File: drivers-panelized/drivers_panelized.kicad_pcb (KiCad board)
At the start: 2 copper layers, 100.9 x 93.6 mm, 583 parts, among them IC1 Motor_A, IC2 Motor_B, J1 Conn_01x07_Pin, J2 Conn_01x07_Pin

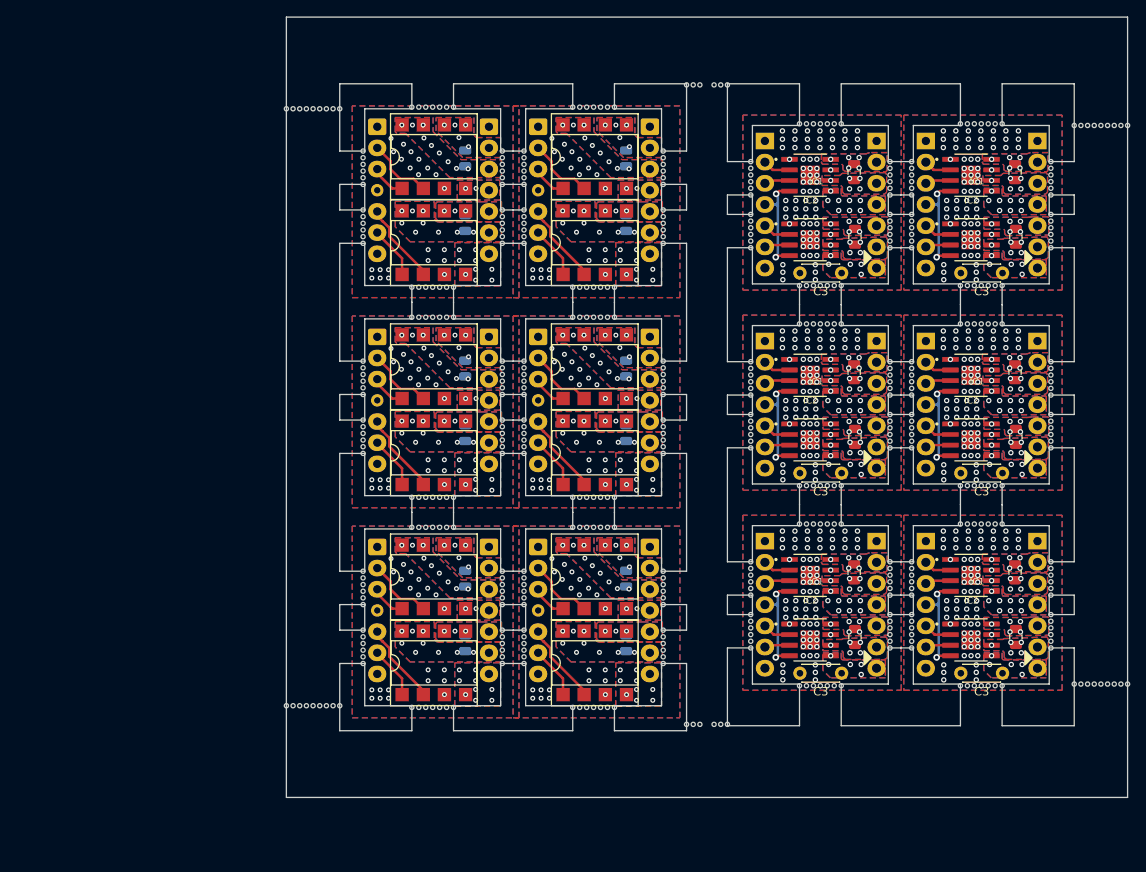
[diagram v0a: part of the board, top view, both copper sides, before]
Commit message: panels again
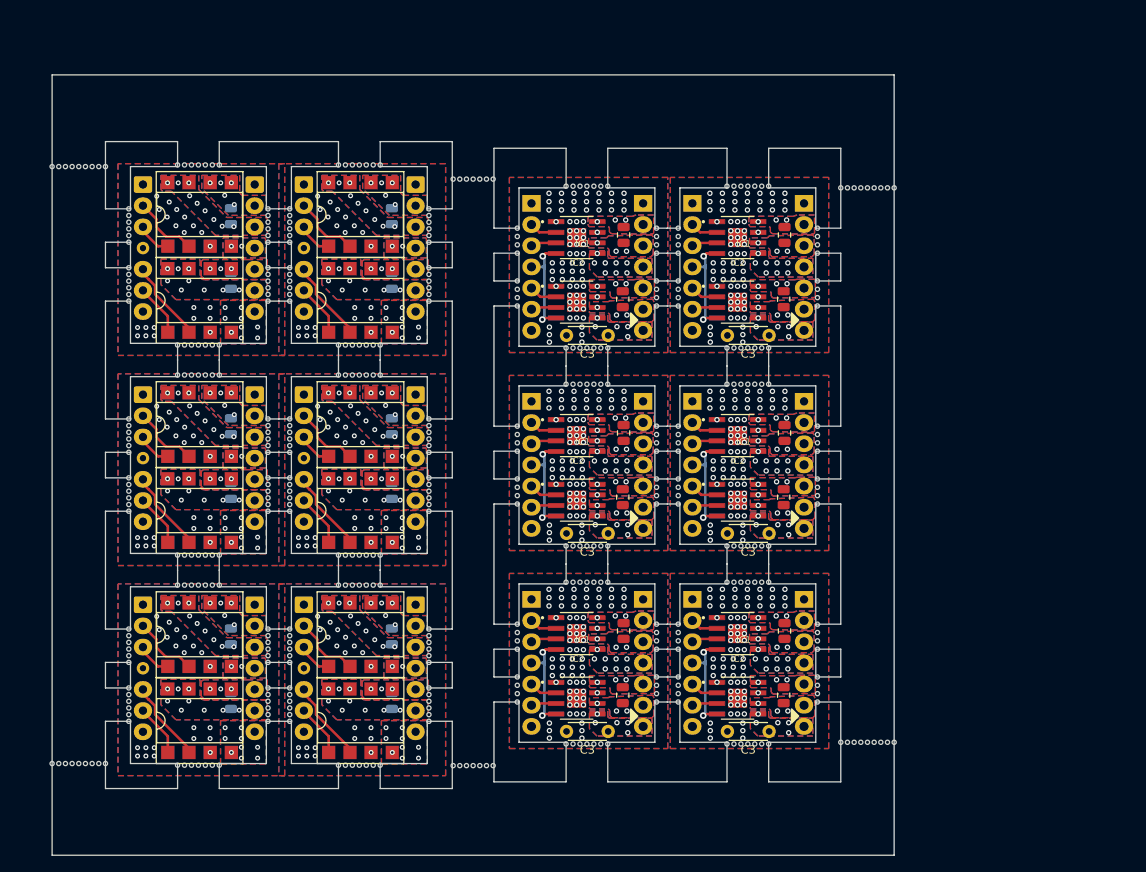
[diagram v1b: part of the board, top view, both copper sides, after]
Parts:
- removed the C1 at (160.3, 97.6)
- removed the C1 at (132.8, 89.4)
- removed the C1 at (113.5, 89.4)
- removed the C1 at (132.8, 64.2)
- removed the C1 at (160.3, 121.6)
- removed the C1 at (179.6, 121.6)
- removed the C1 at (179.6, 73.6)
- removed the C1 at (179.6, 97.6)
- removed the C1 at (160.3, 73.6)
- removed the C1 at (132.8, 114.6)
- removed the C1 at (113.5, 64.2)
- removed the C1 at (113.5, 114.6)
- removed the C2 at (179.5, 65.9)
- removed the C2 at (132.8, 72.0)
- removed the C2 at (113.5, 97.2)
- removed the C2 at (132.8, 97.2)
- removed the C2 at (179.5, 113.9)
- removed the C2 at (179.5, 89.9)
- removed the C2 at (160.2, 89.9)
- removed the C2 at (160.2, 65.9)
- removed the C2 at (160.2, 113.9)
- removed the C2 at (113.5, 122.4)
- removed the C2 at (132.8, 122.4)
- removed the C2 at (113.5, 72.0)
- removed the C3 at (158.7, 78.0)
- removed the C3 at (178.0, 102.0)
- removed the C3 at (178.0, 78.0)
- removed the C3 at (158.7, 126.0)
- removed the C3 at (178.0, 126.0)
- removed the C3 at (158.7, 102.0)
- removed the IC1 at (174.2, 74.0)
- removed the IC1 at (154.9, 74.0)
- removed the IC1 at (174.2, 98.0)
- removed the IC1 at (174.2, 122.0)
- removed the IC1 at (154.9, 98.0)
- removed the IC1 at (154.9, 122.0)
- removed the IC2 at (174.2, 114.2)
- removed the IC2 at (154.9, 90.2)
- removed the IC2 at (174.2, 90.2)
- removed the IC2 at (174.2, 66.2)
- removed the IC2 at (154.9, 114.2)
- removed the IC2 at (154.9, 66.2)
- removed the J1 at (103.0, 60.4)
- removed the J1 at (103.0, 110.8)
- removed the J1 at (149.5, 86.1)
- removed the J1 at (149.5, 110.1)
- removed the J1 at (149.5, 62.1)
- removed the J1 at (168.8, 62.1)
- removed the J1 at (122.3, 60.4)
- removed the J1 at (122.3, 85.6)
- removed the J1 at (168.8, 86.1)
- removed the J1 at (103.0, 85.6)
- removed the J1 at (122.3, 110.8)
- removed the J1 at (168.8, 110.1)
- removed the J2 at (135.7, 85.6)
- removed the J2 at (135.7, 110.8)
- removed the J2 at (162.9, 62.1)
- removed the J2 at (116.4, 85.6)
- removed the J2 at (135.7, 60.4)
- removed the J2 at (162.9, 110.1)
- removed the J2 at (162.9, 86.1)
- removed the J2 at (182.2, 110.1)
- removed the J2 at (182.2, 86.1)
- removed the J2 at (116.4, 60.4)
- removed the J2 at (116.4, 110.8)
- removed the J2 at (182.2, 62.1)
- removed the KiKit_MB_10_1 at (183.8, 70.9)
- removed the KiKit_MB_10_1 at (137.3, 70.4)
- removed the KiKit_MB_10_2 at (183.8, 71.7)
- removed the KiKit_MB_10_2 at (137.3, 71.2)
- removed the KiKit_MB_10_3 at (137.3, 72.0)
- removed the KiKit_MB_10_3 at (183.8, 72.5)
- removed the KiKit_MB_10_4 at (137.3, 72.8)
- removed the KiKit_MB_10_4 at (183.8, 73.3)
- removed the KiKit_MB_10_5 at (137.3, 73.6)
- removed the KiKit_MB_10_5 at (183.8, 74.1)
- removed the KiKit_MB_10_6 at (183.8, 74.9)
- removed the KiKit_MB_10_6 at (137.3, 74.4)
- removed the KiKit_MB_11_1 at (126.5, 58.1)
- removed the KiKit_MB_11_1 at (172.9, 60.1)
- removed the KiKit_MB_11_2 at (173.8, 60.1)
- removed the KiKit_MB_11_2 at (127.3, 58.1)
- removed the KiKit_MB_11_3 at (128.1, 58.1)
- removed the KiKit_MB_11_3 at (174.6, 60.1)
- removed the KiKit_MB_11_4 at (128.9, 58.1)
- removed the KiKit_MB_11_4 at (175.4, 60.1)
- removed the KiKit_MB_11_5 at (129.8, 58.1)
- removed the KiKit_MB_11_5 at (176.3, 60.1)
- removed the KiKit_MB_11_6 at (130.6, 58.1)
- removed the KiKit_MB_11_6 at (177.1, 60.1)
- removed the KiKit_MB_11_7 at (177.9, 60.1)
- removed the KiKit_MB_11_7 at (131.4, 58.1)
- removed the KiKit_MB_12_1 at (131.4, 79.7)
- removed the KiKit_MB_12_1 at (177.9, 79.5)
- removed the KiKit_MB_12_2 at (130.6, 79.7)
- removed the KiKit_MB_12_2 at (177.1, 79.5)
- removed the KiKit_MB_12_3 at (129.8, 79.7)
- removed the KiKit_MB_12_3 at (176.3, 79.5)
- removed the KiKit_MB_12_4 at (175.4, 79.5)
- removed the KiKit_MB_12_4 at (128.9, 79.7)
- removed the KiKit_MB_12_5 at (128.1, 79.7)
- removed the KiKit_MB_12_5 at (174.6, 79.5)
- removed the KiKit_MB_12_6 at (127.3, 79.7)
- removed the KiKit_MB_12_6 at (173.8, 79.5)
- removed the KiKit_MB_12_7 at (126.5, 79.7)
- removed the KiKit_MB_12_7 at (172.9, 79.5)
- removed the KiKit_MB_13_1 at (147.8, 92.6)
- removed the KiKit_MB_13_1 at (101.3, 92.5)
- removed the KiKit_MB_13_2 at (147.8, 91.8)
- removed the KiKit_MB_13_2 at (101.3, 91.7)
- removed the KiKit_MB_13_3 at (101.3, 90.9)
- removed the KiKit_MB_13_3 at (147.8, 91.0)
- removed the KiKit_MB_13_4 at (101.3, 90.1)
- removed the KiKit_MB_13_4 at (147.8, 90.2)
- removed the KiKit_MB_13_5 at (147.8, 89.4)
- removed the KiKit_MB_13_5 at (101.3, 89.3)
- removed the KiKit_MB_13_6 at (101.3, 88.5)
- removed the KiKit_MB_13_6 at (147.8, 88.6)
- removed the KiKit_MB_14_1 at (101.3, 99.6)
- removed the KiKit_MB_14_1 at (147.8, 98.9)
- removed the KiKit_MB_14_2 at (147.8, 98.1)
- removed the KiKit_MB_14_2 at (101.3, 98.8)
- removed the KiKit_MB_14_3 at (101.3, 98.0)
- removed the KiKit_MB_14_3 at (147.8, 97.3)
- removed the KiKit_MB_14_4 at (101.3, 97.2)
- removed the KiKit_MB_14_4 at (147.8, 96.5)
- removed the KiKit_MB_14_5 at (101.3, 96.4)
- removed the KiKit_MB_14_5 at (147.8, 95.7)
- removed the KiKit_MB_14_6 at (147.8, 94.9)
- removed the KiKit_MB_14_6 at (101.3, 95.6)
- removed the KiKit_MB_15_1 at (118.0, 88.5)
- removed the KiKit_MB_15_1 at (164.5, 88.6)
- removed the KiKit_MB_15_2 at (118.0, 89.3)
- removed the KiKit_MB_15_2 at (164.5, 89.4)
- removed the KiKit_MB_15_3 at (164.5, 90.2)
- removed the KiKit_MB_15_3 at (118.0, 90.1)
- removed the KiKit_MB_15_4 at (164.5, 91.0)
- removed the KiKit_MB_15_4 at (118.0, 90.9)
- removed the KiKit_MB_15_5 at (164.5, 91.8)
- removed the KiKit_MB_15_5 at (118.0, 91.7)
- removed the KiKit_MB_15_6 at (118.0, 92.5)
- removed the KiKit_MB_15_6 at (164.5, 92.6)
- removed the KiKit_MB_16_1 at (164.5, 94.9)
- removed the KiKit_MB_16_1 at (118.0, 95.6)
- removed the KiKit_MB_16_2 at (118.0, 96.4)
- removed the KiKit_MB_16_2 at (164.5, 95.7)
- removed the KiKit_MB_16_3 at (164.5, 96.5)
- removed the KiKit_MB_16_3 at (118.0, 97.2)
- removed the KiKit_MB_16_4 at (118.0, 98.0)
- removed the KiKit_MB_16_4 at (164.5, 97.3)
- removed the KiKit_MB_16_5 at (118.0, 98.8)
- removed the KiKit_MB_16_5 at (164.5, 98.1)
- removed the KiKit_MB_16_6 at (118.0, 99.6)
- removed the KiKit_MB_16_6 at (164.5, 98.9)
- removed the KiKit_MB_17_1 at (107.2, 83.3)
- removed the KiKit_MB_17_1 at (153.7, 84.1)
- removed the KiKit_MB_17_2 at (108.0, 83.3)
- removed the KiKit_MB_17_2 at (154.5, 84.1)
- removed the KiKit_MB_17_3 at (108.8, 83.3)
- removed the KiKit_MB_17_3 at (155.3, 84.1)
- removed the KiKit_MB_17_4 at (156.2, 84.1)
- removed the KiKit_MB_17_4 at (109.7, 83.3)
- removed the KiKit_MB_17_5 at (110.5, 83.3)
- removed the KiKit_MB_17_5 at (157.0, 84.1)
- removed the KiKit_MB_17_6 at (111.3, 83.3)
- removed the KiKit_MB_17_6 at (157.8, 84.1)
- removed the KiKit_MB_17_7 at (112.2, 83.3)
- removed the KiKit_MB_17_7 at (158.7, 84.1)
- removed the KiKit_MB_18_1 at (112.2, 104.9)
- removed the KiKit_MB_18_1 at (158.7, 103.5)
- removed the KiKit_MB_18_2 at (111.3, 104.9)
- removed the KiKit_MB_18_2 at (157.8, 103.5)
- removed the KiKit_MB_18_3 at (110.5, 104.9)
- removed the KiKit_MB_18_3 at (157.0, 103.5)
- removed the KiKit_MB_18_4 at (156.2, 103.5)
- removed the KiKit_MB_18_4 at (109.7, 104.9)
- removed the KiKit_MB_18_5 at (155.3, 103.5)
- removed the KiKit_MB_18_5 at (108.8, 104.9)
- removed the KiKit_MB_18_6 at (108.0, 104.9)
- removed the KiKit_MB_18_6 at (154.5, 103.5)
- removed the KiKit_MB_18_7 at (107.2, 104.9)
- removed the KiKit_MB_18_7 at (153.7, 103.5)
- removed the KiKit_MB_19_1 at (167.1, 92.6)
- removed the KiKit_MB_19_1 at (120.6, 92.5)
- removed the KiKit_MB_19_2 at (120.6, 91.7)
- removed the KiKit_MB_19_2 at (167.1, 91.8)
- removed the KiKit_MB_19_3 at (167.1, 91.0)
- removed the KiKit_MB_19_3 at (120.6, 90.9)
- removed the KiKit_MB_19_4 at (167.1, 90.2)
- removed the KiKit_MB_19_4 at (120.6, 90.1)
- removed the KiKit_MB_19_5 at (167.1, 89.4)
- removed the KiKit_MB_19_5 at (120.6, 89.3)
- removed the KiKit_MB_19_6 at (167.1, 88.6)
- removed the KiKit_MB_19_6 at (120.6, 88.5)
- removed the KiKit_MB_1_1 at (101.3, 67.3)
- removed the KiKit_MB_1_1 at (147.8, 68.6)
- removed the KiKit_MB_1_2 at (101.3, 66.5)
- removed the KiKit_MB_1_2 at (147.8, 67.8)
- removed the KiKit_MB_1_3 at (101.3, 65.7)
- removed the KiKit_MB_1_3 at (147.8, 67.0)
- removed the KiKit_MB_1_4 at (101.3, 64.9)
- removed the KiKit_MB_1_4 at (147.8, 66.2)
- removed the KiKit_MB_1_5 at (101.3, 64.1)
- removed the KiKit_MB_1_5 at (147.8, 65.4)
- removed the KiKit_MB_1_6 at (147.8, 64.6)
- removed the KiKit_MB_1_6 at (101.3, 63.3)
- removed the KiKit_MB_20_1 at (120.6, 99.6)
- removed the KiKit_MB_20_1 at (167.1, 98.9)
- removed the KiKit_MB_20_2 at (167.1, 98.1)
- removed the KiKit_MB_20_2 at (120.6, 98.8)
- removed the KiKit_MB_20_3 at (120.6, 98.0)
- removed the KiKit_MB_20_3 at (167.1, 97.3)
- removed the KiKit_MB_20_4 at (120.6, 97.2)
- removed the KiKit_MB_20_4 at (167.1, 96.5)
- removed the KiKit_MB_20_5 at (120.6, 96.4)
- removed the KiKit_MB_20_5 at (167.1, 95.7)
- removed the KiKit_MB_20_6 at (167.1, 94.9)
- removed the KiKit_MB_20_6 at (120.6, 95.6)
- removed the KiKit_MB_21_1 at (183.8, 88.6)
- removed the KiKit_MB_21_1 at (137.3, 88.5)
- removed the KiKit_MB_21_2 at (183.8, 89.4)
- removed the KiKit_MB_21_2 at (137.3, 89.3)
- removed the KiKit_MB_21_3 at (137.3, 90.1)
- removed the KiKit_MB_21_3 at (183.8, 90.2)
- removed the KiKit_MB_21_4 at (183.8, 91.0)
- removed the KiKit_MB_21_4 at (137.3, 90.9)
- removed the KiKit_MB_21_5 at (183.8, 91.8)
- removed the KiKit_MB_21_5 at (137.3, 91.7)
- removed the KiKit_MB_21_6 at (183.8, 92.6)
- removed the KiKit_MB_21_6 at (137.3, 92.5)
- removed the KiKit_MB_22_1 at (183.8, 94.9)
- removed the KiKit_MB_22_1 at (137.3, 95.6)
- removed the KiKit_MB_22_2 at (183.8, 95.7)
- removed the KiKit_MB_22_2 at (137.3, 96.4)
- removed the KiKit_MB_22_3 at (183.8, 96.5)
- removed the KiKit_MB_22_3 at (137.3, 97.2)
- removed the KiKit_MB_22_4 at (137.3, 98.0)
- removed the KiKit_MB_22_4 at (183.8, 97.3)
- removed the KiKit_MB_22_5 at (137.3, 98.8)
- removed the KiKit_MB_22_5 at (183.8, 98.1)
- removed the KiKit_MB_22_6 at (183.8, 98.9)
- removed the KiKit_MB_22_6 at (137.3, 99.6)
- removed the KiKit_MB_23_1 at (172.9, 84.1)
- removed the KiKit_MB_23_1 at (126.5, 83.3)
- removed the KiKit_MB_23_2 at (173.8, 84.1)
- removed the KiKit_MB_23_2 at (127.3, 83.3)
- removed the KiKit_MB_23_3 at (174.6, 84.1)
- removed the KiKit_MB_23_3 at (128.1, 83.3)
- removed the KiKit_MB_23_4 at (175.4, 84.1)
- removed the KiKit_MB_23_4 at (128.9, 83.3)
- removed the KiKit_MB_23_5 at (176.3, 84.1)
- removed the KiKit_MB_23_5 at (129.8, 83.3)
- removed the KiKit_MB_23_6 at (130.6, 83.3)
- removed the KiKit_MB_23_6 at (177.1, 84.1)
- removed the KiKit_MB_23_7 at (131.4, 83.3)
- removed the KiKit_MB_23_7 at (177.9, 84.1)
- removed the KiKit_MB_24_1 at (177.9, 103.5)
- removed the KiKit_MB_24_1 at (131.4, 104.9)
- removed the KiKit_MB_24_2 at (130.6, 104.9)
- removed the KiKit_MB_24_2 at (177.1, 103.5)
- removed the KiKit_MB_24_3 at (129.8, 104.9)
- removed the KiKit_MB_24_3 at (176.3, 103.5)
- removed the KiKit_MB_24_4 at (128.9, 104.9)
- removed the KiKit_MB_24_4 at (175.4, 103.5)
- removed the KiKit_MB_24_5 at (174.6, 103.5)
- removed the KiKit_MB_24_5 at (128.1, 104.9)
- removed the KiKit_MB_24_6 at (127.3, 104.9)
- removed the KiKit_MB_24_6 at (173.8, 103.5)
- removed the KiKit_MB_24_7 at (126.5, 104.9)
- removed the KiKit_MB_24_7 at (172.9, 103.5)
- removed the KiKit_MB_25_1 at (101.3, 117.7)
- removed the KiKit_MB_25_1 at (147.8, 116.6)
- removed the KiKit_MB_25_2 at (147.8, 115.8)
- removed the KiKit_MB_25_2 at (101.3, 116.9)
- removed the KiKit_MB_25_3 at (101.3, 116.1)
- removed the KiKit_MB_25_3 at (147.8, 115.0)
- removed the KiKit_MB_25_4 at (147.8, 114.2)
- removed the KiKit_MB_25_4 at (101.3, 115.3)
- removed the KiKit_MB_25_5 at (101.3, 114.5)
- removed the KiKit_MB_25_5 at (147.8, 113.4)
- removed the KiKit_MB_25_6 at (101.3, 113.7)
- removed the KiKit_MB_25_6 at (147.8, 112.6)
- removed the KiKit_MB_26_1 at (101.3, 124.8)
- removed the KiKit_MB_26_1 at (147.8, 122.9)
- removed the KiKit_MB_26_2 at (147.8, 122.1)
- removed the KiKit_MB_26_2 at (101.3, 124.0)
- removed the KiKit_MB_26_3 at (147.8, 121.3)
- removed the KiKit_MB_26_3 at (101.3, 123.2)
- removed the KiKit_MB_26_4 at (147.8, 120.5)
- removed the KiKit_MB_26_4 at (101.3, 122.4)
- removed the KiKit_MB_26_5 at (147.8, 119.7)
- removed the KiKit_MB_26_5 at (101.3, 121.6)
- removed the KiKit_MB_26_6 at (147.8, 118.9)
- removed the KiKit_MB_26_6 at (101.3, 120.8)
- removed the KiKit_MB_27_1 at (118.0, 113.7)
- removed the KiKit_MB_27_1 at (164.5, 112.6)
- removed the KiKit_MB_27_2 at (164.5, 113.4)
- removed the KiKit_MB_27_2 at (118.0, 114.5)
- removed the KiKit_MB_27_3 at (118.0, 115.3)
- removed the KiKit_MB_27_3 at (164.5, 114.2)
- removed the KiKit_MB_27_4 at (164.5, 115.0)
- removed the KiKit_MB_27_4 at (118.0, 116.1)
- removed the KiKit_MB_27_5 at (164.5, 115.8)
- removed the KiKit_MB_27_5 at (118.0, 116.9)
- removed the KiKit_MB_27_6 at (118.0, 117.7)
- removed the KiKit_MB_27_6 at (164.5, 116.6)
- removed the KiKit_MB_28_1 at (164.5, 118.9)
- removed the KiKit_MB_28_1 at (118.0, 120.8)
- removed the KiKit_MB_28_2 at (164.5, 119.7)
- removed the KiKit_MB_28_2 at (118.0, 121.6)
- removed the KiKit_MB_28_3 at (164.5, 120.5)
- removed the KiKit_MB_28_3 at (118.0, 122.4)
- removed the KiKit_MB_28_4 at (164.5, 121.3)
- removed the KiKit_MB_28_4 at (118.0, 123.2)
- removed the KiKit_MB_28_5 at (118.0, 124.0)
- removed the KiKit_MB_28_5 at (164.5, 122.1)
- removed the KiKit_MB_28_6 at (118.0, 124.8)
- removed the KiKit_MB_28_6 at (164.5, 122.9)
- removed the KiKit_MB_29_1 at (153.7, 108.1)
- removed the KiKit_MB_29_1 at (107.2, 108.5)
- removed the KiKit_MB_29_2 at (108.0, 108.5)
- removed the KiKit_MB_29_2 at (154.5, 108.1)
- removed the KiKit_MB_29_3 at (155.3, 108.1)
- removed the KiKit_MB_29_3 at (108.8, 108.5)
- removed the KiKit_MB_29_4 at (156.2, 108.1)
- removed the KiKit_MB_29_4 at (109.7, 108.5)
- removed the KiKit_MB_29_5 at (110.5, 108.5)
- removed the KiKit_MB_29_5 at (157.0, 108.1)
- removed the KiKit_MB_29_6 at (111.3, 108.5)
- removed the KiKit_MB_29_6 at (157.8, 108.1)
- removed the KiKit_MB_29_7 at (112.2, 108.5)
- removed the KiKit_MB_29_7 at (158.7, 108.1)
- removed the KiKit_MB_2_1 at (101.3, 74.4)
- removed the KiKit_MB_2_1 at (147.8, 74.9)
- removed the KiKit_MB_2_2 at (101.3, 73.6)
- removed the KiKit_MB_2_2 at (147.8, 74.1)
- removed the KiKit_MB_2_3 at (101.3, 72.8)
- removed the KiKit_MB_2_3 at (147.8, 73.3)
- removed the KiKit_MB_2_4 at (101.3, 72.0)
- removed the KiKit_MB_2_4 at (147.8, 72.5)
- removed the KiKit_MB_2_5 at (101.3, 71.2)
- removed the KiKit_MB_2_5 at (147.8, 71.7)
- removed the KiKit_MB_2_6 at (101.3, 70.4)
- removed the KiKit_MB_2_6 at (147.8, 70.9)
- removed the KiKit_MB_30_1 at (158.7, 127.5)
- removed the KiKit_MB_30_1 at (112.2, 130.1)
- removed the KiKit_MB_30_2 at (111.3, 130.1)
- removed the KiKit_MB_30_2 at (157.8, 127.5)
- removed the KiKit_MB_30_3 at (110.5, 130.1)
- removed the KiKit_MB_30_3 at (157.0, 127.5)
- removed the KiKit_MB_30_4 at (109.7, 130.1)
- removed the KiKit_MB_30_4 at (156.2, 127.5)
- removed the KiKit_MB_30_5 at (108.8, 130.1)
- removed the KiKit_MB_30_5 at (155.3, 127.5)
- removed the KiKit_MB_30_6 at (154.5, 127.5)
- removed the KiKit_MB_30_6 at (108.0, 130.1)
- removed the KiKit_MB_30_7 at (153.7, 127.5)
- removed the KiKit_MB_30_7 at (107.2, 130.1)
- removed the KiKit_MB_31_1 at (120.6, 117.7)
- removed the KiKit_MB_31_1 at (167.1, 116.6)
- removed the KiKit_MB_31_2 at (120.6, 116.9)
- removed the KiKit_MB_31_2 at (167.1, 115.8)
- removed the KiKit_MB_31_3 at (120.6, 116.1)
- removed the KiKit_MB_31_3 at (167.1, 115.0)
- removed the KiKit_MB_31_4 at (120.6, 115.3)
- removed the KiKit_MB_31_4 at (167.1, 114.2)
- removed the KiKit_MB_31_5 at (120.6, 114.5)
- removed the KiKit_MB_31_5 at (167.1, 113.4)
- removed the KiKit_MB_31_6 at (167.1, 112.6)
- removed the KiKit_MB_31_6 at (120.6, 113.7)
- removed the KiKit_MB_32_1 at (120.6, 124.8)
- removed the KiKit_MB_32_1 at (167.1, 122.9)
- removed the KiKit_MB_32_2 at (167.1, 122.1)
- removed the KiKit_MB_32_2 at (120.6, 124.0)
- removed the KiKit_MB_32_3 at (167.1, 121.3)
- removed the KiKit_MB_32_3 at (120.6, 123.2)
- removed the KiKit_MB_32_4 at (120.6, 122.4)
- removed the KiKit_MB_32_4 at (167.1, 120.5)
- removed the KiKit_MB_32_5 at (167.1, 119.7)
- removed the KiKit_MB_32_5 at (120.6, 121.6)
- removed the KiKit_MB_32_6 at (167.1, 118.9)
- removed the KiKit_MB_32_6 at (120.6, 120.8)
- removed the KiKit_MB_33_1 at (183.8, 112.6)
- removed the KiKit_MB_33_1 at (137.3, 113.7)
- removed the KiKit_MB_33_2 at (183.8, 113.4)
- removed the KiKit_MB_33_2 at (137.3, 114.5)
- removed the KiKit_MB_33_3 at (183.8, 114.2)
- removed the KiKit_MB_33_3 at (137.3, 115.3)
- removed the KiKit_MB_33_4 at (137.3, 116.1)
- removed the KiKit_MB_33_4 at (183.8, 115.0)
- removed the KiKit_MB_33_5 at (183.8, 115.8)
- removed the KiKit_MB_33_5 at (137.3, 116.9)
- removed the KiKit_MB_33_6 at (137.3, 117.7)
- removed the KiKit_MB_33_6 at (183.8, 116.6)
- removed the KiKit_MB_34_1 at (137.3, 120.8)
- removed the KiKit_MB_34_1 at (183.8, 118.9)
- removed the KiKit_MB_34_2 at (183.8, 119.7)
- removed the KiKit_MB_34_2 at (137.3, 121.6)
- removed the KiKit_MB_34_3 at (183.8, 120.5)
- removed the KiKit_MB_34_3 at (137.3, 122.4)
- removed the KiKit_MB_34_4 at (137.3, 123.2)
- removed the KiKit_MB_34_4 at (183.8, 121.3)
- removed the KiKit_MB_34_5 at (183.8, 122.1)
- removed the KiKit_MB_34_5 at (137.3, 124.0)
- removed the KiKit_MB_34_6 at (183.8, 122.9)
- removed the KiKit_MB_34_6 at (137.3, 124.8)
- removed the KiKit_MB_35_1 at (126.5, 108.5)
- removed the KiKit_MB_35_1 at (172.9, 108.1)
- removed the KiKit_MB_35_2 at (127.3, 108.5)
- removed the KiKit_MB_35_2 at (173.8, 108.1)
- removed the KiKit_MB_35_3 at (174.6, 108.1)
- removed the KiKit_MB_35_3 at (128.1, 108.5)
- removed the KiKit_MB_35_4 at (175.4, 108.1)
- removed the KiKit_MB_35_4 at (128.9, 108.5)
- removed the KiKit_MB_35_5 at (129.8, 108.5)
- removed the KiKit_MB_35_5 at (176.3, 108.1)
- removed the KiKit_MB_35_6 at (130.6, 108.5)
- removed the KiKit_MB_35_6 at (177.1, 108.1)
- removed the KiKit_MB_35_7 at (131.4, 108.5)
- removed the KiKit_MB_35_7 at (177.9, 108.1)
- removed the KiKit_MB_36_1 at (131.4, 130.1)
- removed the KiKit_MB_36_1 at (177.9, 127.5)
- removed the KiKit_MB_36_2 at (177.1, 127.5)
- removed the KiKit_MB_36_2 at (130.6, 130.1)
- removed the KiKit_MB_36_3 at (176.3, 127.5)
- removed the KiKit_MB_36_3 at (129.8, 130.1)
- removed the KiKit_MB_36_4 at (128.9, 130.1)
- removed the KiKit_MB_36_4 at (175.4, 127.5)
- removed the KiKit_MB_36_5 at (128.1, 130.1)
- removed the KiKit_MB_36_5 at (174.6, 127.5)
- removed the KiKit_MB_36_6 at (173.8, 127.5)
- removed the KiKit_MB_36_6 at (127.3, 130.1)
- removed the KiKit_MB_36_7 at (172.9, 127.5)
- removed the KiKit_MB_36_7 at (126.5, 130.1)
- removed the KiKit_MB_37_10 at (97.7, 58.3)
- removed the KiKit_MB_37_4 at (92.9, 58.3)
- removed the KiKit_MB_37_5 at (93.7, 58.3)
- removed the KiKit_MB_37_6 at (94.5, 58.3)
- removed the KiKit_MB_37_7 at (95.3, 58.3)
- removed the KiKit_MB_37_8 at (96.1, 58.3)
- removed the KiKit_MB_37_9 at (96.9, 58.3)
- removed the KiKit_MB_3_1 at (164.5, 64.6)
- removed the KiKit_MB_3_1 at (118.0, 63.3)
- removed the KiKit_MB_3_2 at (164.5, 65.4)
- removed the KiKit_MB_3_2 at (118.0, 64.1)
- removed the KiKit_MB_3_3 at (118.0, 64.9)
- removed the KiKit_MB_3_3 at (164.5, 66.2)
- removed the KiKit_MB_3_4 at (164.5, 67.0)
- removed the KiKit_MB_3_4 at (118.0, 65.7)
- removed the KiKit_MB_3_5 at (164.5, 67.8)
- removed the KiKit_MB_3_5 at (118.0, 66.5)
- removed the KiKit_MB_3_6 at (164.5, 68.6)
- removed the KiKit_MB_3_6 at (118.0, 67.3)
- removed the KiKit_MB_40_1 at (186.6, 127.3)
- removed the KiKit_MB_40_1 at (140.1, 55.4)
- removed the KiKit_MB_40_1 at (140.1, 132.1)
- removed KiKit_MB_40_10 (x2), KiKit_MB_40_11 (x2): NPTH, NPTH
- removed the KiKit_MB_40_2 at (187.4, 127.3)
- removed the KiKit_MB_40_2 at (140.9, 55.4)
- removed the KiKit_MB_40_2 at (140.9, 132.1)
- removed the KiKit_MB_40_3 at (188.2, 127.3)
- removed the KiKit_MB_40_3 at (141.7, 55.4)
- removed the KiKit_MB_40_3 at (141.7, 132.1)
- removed the KiKit_MB_40_9 at (143.4, 132.1)
- removed the KiKit_MB_40_9 at (143.4, 55.4)
- removed the KiKit_MB_40_9 at (193.0, 127.3)
- removed the KiKit_MB_4_1 at (118.0, 70.4)
- removed the KiKit_MB_4_1 at (164.5, 70.9)
- removed the KiKit_MB_4_2 at (164.5, 71.7)
- removed the KiKit_MB_4_2 at (118.0, 71.2)
- removed the KiKit_MB_4_3 at (118.0, 72.0)
- removed the KiKit_MB_4_3 at (164.5, 72.5)
- removed the KiKit_MB_4_4 at (118.0, 72.8)
- removed the KiKit_MB_4_4 at (164.5, 73.3)
- removed the KiKit_MB_4_5 at (118.0, 73.6)
- removed the KiKit_MB_4_5 at (164.5, 74.1)
- removed the KiKit_MB_4_6 at (118.0, 74.4)
- removed the KiKit_MB_4_6 at (164.5, 74.9)
- removed the KiKit_MB_5_1 at (107.2, 58.1)
- removed the KiKit_MB_5_1 at (153.7, 60.1)
- removed the KiKit_MB_5_2 at (154.5, 60.1)
- removed the KiKit_MB_5_2 at (108.0, 58.1)
- removed the KiKit_MB_5_3 at (155.3, 60.1)
- removed the KiKit_MB_5_3 at (108.8, 58.1)
- removed the KiKit_MB_5_4 at (156.2, 60.1)
- removed the KiKit_MB_5_4 at (109.7, 58.1)
- removed the KiKit_MB_5_5 at (110.5, 58.1)
- removed the KiKit_MB_5_5 at (157.0, 60.1)
- removed the KiKit_MB_5_6 at (157.8, 60.1)
- removed the KiKit_MB_5_6 at (111.3, 58.1)
- removed the KiKit_MB_5_7 at (158.7, 60.1)
- removed the KiKit_MB_5_7 at (112.2, 58.1)
- removed the KiKit_MB_6_1 at (158.7, 79.5)
- removed the KiKit_MB_6_1 at (112.2, 79.7)
- removed the KiKit_MB_6_2 at (157.8, 79.5)
- removed the KiKit_MB_6_2 at (111.3, 79.7)
- removed the KiKit_MB_6_3 at (157.0, 79.5)
- removed the KiKit_MB_6_3 at (110.5, 79.7)
- removed the KiKit_MB_6_4 at (156.2, 79.5)
- removed the KiKit_MB_6_4 at (109.7, 79.7)
- removed the KiKit_MB_6_5 at (108.8, 79.7)
- removed the KiKit_MB_6_5 at (155.3, 79.5)
- removed the KiKit_MB_6_6 at (154.5, 79.5)
- removed the KiKit_MB_6_6 at (108.0, 79.7)
- removed the KiKit_MB_6_7 at (153.7, 79.5)
- removed the KiKit_MB_6_7 at (107.2, 79.7)
- removed the KiKit_MB_7_1 at (167.1, 68.6)
- removed the KiKit_MB_7_1 at (120.6, 67.3)
- removed the KiKit_MB_7_2 at (167.1, 67.8)
- removed the KiKit_MB_7_2 at (120.6, 66.5)
- removed the KiKit_MB_7_3 at (120.6, 65.7)
- removed the KiKit_MB_7_3 at (167.1, 67.0)
- removed the KiKit_MB_7_4 at (167.1, 66.2)
- removed the KiKit_MB_7_4 at (120.6, 64.9)
- removed the KiKit_MB_7_5 at (120.6, 64.1)
- removed the KiKit_MB_7_5 at (167.1, 65.4)
- removed the KiKit_MB_7_6 at (120.6, 63.3)
- removed the KiKit_MB_7_6 at (167.1, 64.6)
- removed the KiKit_MB_8_1 at (167.1, 74.9)
- removed the KiKit_MB_8_1 at (120.6, 74.4)
- removed the KiKit_MB_8_2 at (167.1, 74.1)
- removed the KiKit_MB_8_2 at (120.6, 73.6)
- removed the KiKit_MB_8_3 at (167.1, 73.3)
- removed the KiKit_MB_8_3 at (120.6, 72.8)
- removed the KiKit_MB_8_4 at (120.6, 72.0)
- removed the KiKit_MB_8_4 at (167.1, 72.5)
- removed the KiKit_MB_8_5 at (120.6, 71.2)
- removed the KiKit_MB_8_5 at (167.1, 71.7)
- removed the KiKit_MB_8_6 at (167.1, 70.9)
- removed the KiKit_MB_8_6 at (120.6, 70.4)
- removed the KiKit_MB_9_1 at (137.3, 63.3)
- removed the KiKit_MB_9_1 at (183.8, 64.6)
- removed the KiKit_MB_9_2 at (183.8, 65.4)
- removed the KiKit_MB_9_2 at (137.3, 64.1)
- removed the KiKit_MB_9_3 at (183.8, 66.2)
- removed the KiKit_MB_9_3 at (137.3, 64.9)
- removed the KiKit_MB_9_4 at (137.3, 65.7)
- removed the KiKit_MB_9_4 at (183.8, 67.0)
- removed the KiKit_MB_9_5 at (183.8, 67.8)
- removed the KiKit_MB_9_5 at (137.3, 66.5)
- removed the KiKit_MB_9_6 at (183.8, 68.6)
- removed the KiKit_MB_9_6 at (137.3, 67.3)
- removed the U1 at (109.8, 74.3)
- removed the U1 at (129.1, 124.7)
- removed the U1 at (109.8, 99.5)
- removed the U1 at (129.1, 99.5)
- removed the U1 at (109.8, 124.7)
- removed the U1 at (129.1, 74.3)
- removed the U2 at (129.1, 89.2)
- removed the U2 at (129.1, 64.0)
- removed the U2 at (129.1, 114.4)
- removed the U2 at (109.8, 89.2)
- removed the U2 at (109.8, 114.4)
- removed the U2 at (109.8, 64.0)
- added C1: 100n, Capacitor_SMD:C_0805_2012Metric, F.Cu at (151.8, 120.9)
- added C1: 100, Capacitor_SMD:C_0805_2012Metric, B.Cu at (85.5, 71.2)
- added C1: 100, Capacitor_SMD:C_0805_2012Metric, B.Cu at (104.8, 96.3)
- added C1: 100, Capacitor_SMD:C_0805_2012Metric, B.Cu at (85.5, 121.5)
- added C1: 100n, Capacitor_SMD:C_0805_2012Metric, F.Cu at (151.8, 97.2)
- added C1: 100n, Capacitor_SMD:C_0805_2012Metric, F.Cu at (132.6, 120.9)
- added C1: 100n, Capacitor_SMD:C_0805_2012Metric, F.Cu at (132.6, 73.4)
- added C1: 100n, Capacitor_SMD:C_0805_2012Metric, F.Cu at (151.8, 73.4)
- added C1: 100n, Capacitor_SMD:C_0805_2012Metric, F.Cu at (132.6, 97.2)
- added C1: 100, Capacitor_SMD:C_0805_2012Metric, B.Cu at (104.8, 121.5)
- added C1: 100, Capacitor_SMD:C_0805_2012Metric, B.Cu at (85.5, 96.3)
- added C1: 100, Capacitor_SMD:C_0805_2012Metric, B.Cu at (104.8, 71.2)
- added C2: 100n, Capacitor_SMD:C_0805_2012Metric, F.Cu at (132.4, 81.1)
- added C2: 100, Capacitor_SMD:C_0805_2012Metric, B.Cu at (104.8, 78.9)
- added C2: 100, Capacitor_SMD:C_0805_2012Metric, B.Cu at (85.5, 78.9)
- added C2: 100, Capacitor_SMD:C_0805_2012Metric, B.Cu at (104.8, 104.1)
- added C2: 100n, Capacitor_SMD:C_0805_2012Metric, F.Cu at (132.4, 104.8)
- added C2: 100n, Capacitor_SMD:C_0805_2012Metric, F.Cu at (151.8, 128.6)
- added C2: 100n, Capacitor_SMD:C_0805_2012Metric, F.Cu at (151.8, 81.1)
- added C2: 100n, Capacitor_SMD:C_0805_2012Metric, F.Cu at (132.4, 128.6)
- added C2: 100n, Capacitor_SMD:C_0805_2012Metric, F.Cu at (151.8, 104.8)
- added C2: 100, Capacitor_SMD:C_0805_2012Metric, B.Cu at (104.8, 129.3)
- added C2: 100, Capacitor_SMD:C_0805_2012Metric, B.Cu at (85.5, 104.1)
- added C2: 100, Capacitor_SMD:C_0805_2012Metric, B.Cu at (85.5, 129.3)
- added C3: 100u, Capacitor_THT:C_Disc_D4.3mm_W1.9mm_P5.00mm, F.Cu at (130.7, 85.5)
- added C3: 100u, Capacitor_THT:C_Disc_D4.3mm_W1.9mm_P5.00mm, F.Cu at (150.0, 109.2)
- added C3: 100u, Capacitor_THT:C_Disc_D4.3mm_W1.9mm_P5.00mm, F.Cu at (150.0, 132.9)
- added C3: 100u, Capacitor_THT:C_Disc_D4.3mm_W1.9mm_P5.00mm, F.Cu at (130.7, 132.9)
- added C3: 100u, Capacitor_THT:C_Disc_D4.3mm_W1.9mm_P5.00mm, F.Cu at (130.7, 109.2)
- added C3: 100u, Capacitor_THT:C_Disc_D4.3mm_W1.9mm_P5.00mm, F.Cu at (150.0, 85.5)
- added IC1: Motor_A, TB67H450FNG_EL:TB67H450FNG_EL, F.Cu at (146.2, 129.0)
- added IC1: Motor_A, TB67H450FNG_EL:TB67H450FNG_EL, F.Cu at (146.2, 105.2)
- added IC1: Motor_A, TB67H450FNG_EL:TB67H450FNG_EL, F.Cu at (126.9, 129.0)
- added IC1: Motor_A, TB67H450FNG_EL:TB67H450FNG_EL, F.Cu at (126.9, 105.2)
- added IC1: Motor_A, TB67H450FNG_EL:TB67H450FNG_EL, F.Cu at (146.2, 81.5)
- added IC1: Motor_A, TB67H450FNG_EL:TB67H450FNG_EL, F.Cu at (126.9, 81.5)
- added IC2: Motor_B, TB67H450FNG_EL:TB67H450FNG_EL, F.Cu at (126.9, 97.5)
- added IC2: Motor_B, TB67H450FNG_EL:TB67H450FNG_EL, F.Cu at (146.2, 97.5)
- added IC2: Motor_B, TB67H450FNG_EL:TB67H450FNG_EL, F.Cu at (146.2, 73.7)
- added IC2: Motor_B, TB67H450FNG_EL:TB67H450FNG_EL, F.Cu at (146.2, 121.2)
- added IC2: Motor_B, TB67H450FNG_EL:TB67H450FNG_EL, F.Cu at (126.9, 73.7)
- added IC2: Motor_B, TB67H450FNG_EL:TB67H450FNG_EL, F.Cu at (126.9, 121.2)
- added J1: Conn_01x07_Pin, Connector_PinHeader_2.54mm:PinHeader_1x07_P2.54mm_Vertical, B.Cu at (121.5, 93.4)
- added J1: Conn_01x07_Pin, Connector_PinHeader_2.54mm:PinHeader_1x07_P2.54mm_Vertical, B.Cu at (94.2, 67.3)
- added J1: Conn_01x07_Pin, Connector_PinHeader_2.54mm:PinHeader_1x07_P2.54mm_Vertical, B.Cu at (94.2, 92.5)
- added J1: Conn_01x07_Pin, Connector_PinHeader_2.54mm:PinHeader_1x07_P2.54mm_Vertical, B.Cu at (121.5, 69.6)
- added J1: Conn_01x07_Pin, Connector_PinHeader_2.54mm:PinHeader_1x07_P2.54mm_Vertical, B.Cu at (74.9, 67.3)
- added J1: Conn_01x07_Pin, Connector_PinHeader_2.54mm:PinHeader_1x07_P2.54mm_Vertical, B.Cu at (140.8, 93.4)
- added J1: Conn_01x07_Pin, Connector_PinHeader_2.54mm:PinHeader_1x07_P2.54mm_Vertical, B.Cu at (74.9, 117.8)
- added J1: Conn_01x07_Pin, Connector_PinHeader_2.54mm:PinHeader_1x07_P2.54mm_Vertical, B.Cu at (121.5, 117.1)
- added J1: Conn_01x07_Pin, Connector_PinHeader_2.54mm:PinHeader_1x07_P2.54mm_Vertical, B.Cu at (74.9, 92.5)
- added J1: Conn_01x07_Pin, Connector_PinHeader_2.54mm:PinHeader_1x07_P2.54mm_Vertical, B.Cu at (140.8, 69.6)
- added J1: Conn_01x07_Pin, Connector_PinHeader_2.54mm:PinHeader_1x07_P2.54mm_Vertical, B.Cu at (94.2, 117.8)
- added J1: Conn_01x07_Pin, Connector_PinHeader_2.54mm:PinHeader_1x07_P2.54mm_Vertical, B.Cu at (140.8, 117.1)
- added J2: Conn_01x07_Pin, Connector_PinHeader_2.54mm:PinHeader_1x07_P2.54mm_Vertical, B.Cu at (107.6, 117.8)
- added J2: Conn_01x07_Pin, Connector_PinHeader_2.54mm:PinHeader_1x07_P2.54mm_Vertical, B.Cu at (134.9, 117.1)
- added J2: Conn_01x07_Pin, Connector_PinHeader_2.54mm:PinHeader_1x07_P2.54mm_Vertical, B.Cu at (134.9, 93.4)
- added J2: Conn_01x07_Pin, Connector_PinHeader_2.54mm:PinHeader_1x07_P2.54mm_Vertical, B.Cu at (88.3, 92.5)
- added J2: Conn_01x07_Pin, Connector_PinHeader_2.54mm:PinHeader_1x07_P2.54mm_Vertical, B.Cu at (134.9, 69.6)
- added J2: Conn_01x07_Pin, Connector_PinHeader_2.54mm:PinHeader_1x07_P2.54mm_Vertical, B.Cu at (154.2, 69.6)
- added J2: Conn_01x07_Pin, Connector_PinHeader_2.54mm:PinHeader_1x07_P2.54mm_Vertical, B.Cu at (154.2, 93.4)
- added J2: Conn_01x07_Pin, Connector_PinHeader_2.54mm:PinHeader_1x07_P2.54mm_Vertical, B.Cu at (107.6, 67.3)
- added J2: Conn_01x07_Pin, Connector_PinHeader_2.54mm:PinHeader_1x07_P2.54mm_Vertical, B.Cu at (88.3, 117.8)
- added J2: Conn_01x07_Pin, Connector_PinHeader_2.54mm:PinHeader_1x07_P2.54mm_Vertical, B.Cu at (154.2, 117.1)
- added J2: Conn_01x07_Pin, Connector_PinHeader_2.54mm:PinHeader_1x07_P2.54mm_Vertical, B.Cu at (107.6, 92.5)
- added J2: Conn_01x07_Pin, Connector_PinHeader_2.54mm:PinHeader_1x07_P2.54mm_Vertical, B.Cu at (88.3, 67.3)
- added KiKit_MB_10_1: NPTH, NPTH, F.Cu at (109.2, 77.3)
- added KiKit_MB_10_1: NPTH, NPTH, F.Cu at (155.8, 78.9)
- added KiKit_MB_10_2: NPTH, NPTH, F.Cu at (109.2, 78.1)
- added KiKit_MB_10_2: NPTH, NPTH, F.Cu at (155.8, 79.9)
- added KiKit_MB_10_3: NPTH, NPTH, F.Cu at (155.8, 80.9)
- added KiKit_MB_10_3: NPTH, NPTH, F.Cu at (109.2, 78.9)
- added KiKit_MB_10_4: NPTH, NPTH, F.Cu at (155.8, 81.9)
- added KiKit_MB_10_4: NPTH, NPTH, F.Cu at (109.2, 79.7)
- added KiKit_MB_10_5: NPTH, NPTH, F.Cu at (109.2, 80.5)
- added KiKit_MB_10_6: NPTH, NPTH, F.Cu at (109.2, 81.3)
- added KiKit_MB_11_1: NPTH, NPTH, F.Cu at (98.3, 65.0)
- added KiKit_MB_11_1: NPTH, NPTH, F.Cu at (144.9, 67.5)
- added KiKit_MB_11_2: NPTH, NPTH, F.Cu at (99.2, 65.0)
- added KiKit_MB_11_2: NPTH, NPTH, F.Cu at (145.8, 67.5)
- added KiKit_MB_11_3: NPTH, NPTH, F.Cu at (100.0, 65.0)
- added KiKit_MB_11_3: NPTH, NPTH, F.Cu at (146.6, 67.5)
- added KiKit_MB_11_4: NPTH, NPTH, F.Cu at (100.8, 65.0)
- added KiKit_MB_11_4: NPTH, NPTH, F.Cu at (147.4, 67.5)
- added KiKit_MB_11_5: NPTH, NPTH, F.Cu at (101.7, 65.0)
- added KiKit_MB_11_5: NPTH, NPTH, F.Cu at (148.3, 67.5)
- added KiKit_MB_11_6: NPTH, NPTH, F.Cu at (149.1, 67.5)
- added KiKit_MB_11_6: NPTH, NPTH, F.Cu at (102.5, 65.0)
- added KiKit_MB_11_7: NPTH, NPTH, F.Cu at (149.9, 67.5)
- added KiKit_MB_11_7: NPTH, NPTH, F.Cu at (103.3, 65.0)
- added KiKit_MB_12_1: NPTH, NPTH, F.Cu at (103.3, 86.6)
- added KiKit_MB_12_1: NPTH, NPTH, F.Cu at (149.9, 87.0)
- added KiKit_MB_12_2: NPTH, NPTH, F.Cu at (102.5, 86.6)
- added KiKit_MB_12_2: NPTH, NPTH, F.Cu at (149.1, 87.0)
- added KiKit_MB_12_3: NPTH, NPTH, F.Cu at (148.3, 87.0)
- added KiKit_MB_12_3: NPTH, NPTH, F.Cu at (101.7, 86.6)
- added KiKit_MB_12_4: NPTH, NPTH, F.Cu at (147.4, 87.0)
- added KiKit_MB_12_4: NPTH, NPTH, F.Cu at (100.8, 86.6)
- added KiKit_MB_12_5: NPTH, NPTH, F.Cu at (146.6, 87.0)
- added KiKit_MB_12_5: NPTH, NPTH, F.Cu at (100.0, 86.6)
- added KiKit_MB_12_6: NPTH, NPTH, F.Cu at (145.8, 87.0)
- added KiKit_MB_12_6: NPTH, NPTH, F.Cu at (99.2, 86.6)
- added KiKit_MB_12_7: NPTH, NPTH, F.Cu at (144.9, 87.0)
- added KiKit_MB_12_7: NPTH, NPTH, F.Cu at (98.3, 86.6)
- added KiKit_MB_13_1: NPTH, NPTH, F.Cu at (73.2, 99.5)
- added KiKit_MB_13_1: NPTH, NPTH, F.Cu at (119.8, 99.3)
- added KiKit_MB_13_2: NPTH, NPTH, F.Cu at (73.2, 98.7)
- added KiKit_MB_13_2: NPTH, NPTH, F.Cu at (119.8, 98.3)
- added KiKit_MB_13_3: NPTH, NPTH, F.Cu at (119.8, 97.3)
- added KiKit_MB_13_3: NPTH, NPTH, F.Cu at (73.2, 97.9)
- added KiKit_MB_13_4: NPTH, NPTH, F.Cu at (119.8, 96.3)
- added KiKit_MB_13_4: NPTH, NPTH, F.Cu at (73.2, 97.1)
- added KiKit_MB_13_5: NPTH, NPTH, F.Cu at (73.2, 96.3)
- added KiKit_MB_13_6: NPTH, NPTH, F.Cu at (73.2, 95.5)
- added KiKit_MB_14_1: NPTH, NPTH, F.Cu at (73.2, 106.5)
- added KiKit_MB_14_1: NPTH, NPTH, F.Cu at (119.8, 105.7)
- added KiKit_MB_14_2: NPTH, NPTH, F.Cu at (119.8, 104.7)
- added KiKit_MB_14_2: NPTH, NPTH, F.Cu at (73.2, 105.7)
- added KiKit_MB_14_3: NPTH, NPTH, F.Cu at (119.8, 103.7)
- added KiKit_MB_14_3: NPTH, NPTH, F.Cu at (73.2, 104.9)
- added KiKit_MB_14_4: NPTH, NPTH, F.Cu at (73.2, 104.1)
- added KiKit_MB_14_4: NPTH, NPTH, F.Cu at (119.8, 102.7)
- added KiKit_MB_14_5: NPTH, NPTH, F.Cu at (73.2, 103.3)
- added KiKit_MB_14_6: NPTH, NPTH, F.Cu at (73.2, 102.5)
- added KiKit_MB_15_1: NPTH, NPTH, F.Cu at (136.5, 96.3)
- added KiKit_MB_15_1: NPTH, NPTH, F.Cu at (89.9, 95.5)
- added KiKit_MB_15_2: NPTH, NPTH, F.Cu at (89.9, 96.3)
- added KiKit_MB_15_2: NPTH, NPTH, F.Cu at (136.5, 97.3)
- added KiKit_MB_15_3: NPTH, NPTH, F.Cu at (89.9, 97.1)
- added KiKit_MB_15_3: NPTH, NPTH, F.Cu at (136.5, 98.3)
- added KiKit_MB_15_4: NPTH, NPTH, F.Cu at (136.5, 99.3)
- added KiKit_MB_15_4: NPTH, NPTH, F.Cu at (89.9, 97.9)
- added KiKit_MB_15_5: NPTH, NPTH, F.Cu at (89.9, 98.7)
- added KiKit_MB_15_6: NPTH, NPTH, F.Cu at (89.9, 99.5)
- added KiKit_MB_16_1: NPTH, NPTH, F.Cu at (136.5, 102.7)
- added KiKit_MB_16_1: NPTH, NPTH, F.Cu at (89.9, 102.5)
- added KiKit_MB_16_2: NPTH, NPTH, F.Cu at (89.9, 103.3)
- added KiKit_MB_16_2: NPTH, NPTH, F.Cu at (136.5, 103.7)
- added KiKit_MB_16_3: NPTH, NPTH, F.Cu at (136.5, 104.7)
- added KiKit_MB_16_3: NPTH, NPTH, F.Cu at (89.9, 104.1)
- added KiKit_MB_16_4: NPTH, NPTH, F.Cu at (136.5, 105.7)
- added KiKit_MB_16_4: NPTH, NPTH, F.Cu at (89.9, 104.9)
- added KiKit_MB_16_5: NPTH, NPTH, F.Cu at (89.9, 105.7)
- added KiKit_MB_16_6: NPTH, NPTH, F.Cu at (89.9, 106.5)
- added KiKit_MB_17_1: NPTH, NPTH, F.Cu at (79.0, 90.2)
- added KiKit_MB_17_1: NPTH, NPTH, F.Cu at (125.7, 91.3)
- added KiKit_MB_17_2: NPTH, NPTH, F.Cu at (79.9, 90.2)
- added KiKit_MB_17_2: NPTH, NPTH, F.Cu at (126.5, 91.3)
- added KiKit_MB_17_3: NPTH, NPTH, F.Cu at (127.3, 91.3)
- added KiKit_MB_17_3: NPTH, NPTH, F.Cu at (80.7, 90.2)
- added KiKit_MB_17_4: NPTH, NPTH, F.Cu at (81.5, 90.2)
- added KiKit_MB_17_4: NPTH, NPTH, F.Cu at (128.2, 91.3)
- added KiKit_MB_17_5: NPTH, NPTH, F.Cu at (82.4, 90.2)
- added KiKit_MB_17_5: NPTH, NPTH, F.Cu at (129.0, 91.3)
- added KiKit_MB_17_6: NPTH, NPTH, F.Cu at (129.8, 91.3)
- added KiKit_MB_17_6: NPTH, NPTH, F.Cu at (83.2, 90.2)
- added KiKit_MB_17_7: NPTH, NPTH, F.Cu at (84.0, 90.2)
- added KiKit_MB_17_7: NPTH, NPTH, F.Cu at (130.7, 91.3)
- added KiKit_MB_18_1: NPTH, NPTH, F.Cu at (84.0, 111.8)
- added KiKit_MB_18_1: NPTH, NPTH, F.Cu at (130.7, 110.7)
- added KiKit_MB_18_2: NPTH, NPTH, F.Cu at (129.8, 110.7)
- added KiKit_MB_18_2: NPTH, NPTH, F.Cu at (83.2, 111.8)
- added KiKit_MB_18_3: NPTH, NPTH, F.Cu at (129.0, 110.7)
- added KiKit_MB_18_3: NPTH, NPTH, F.Cu at (82.4, 111.8)
- added KiKit_MB_18_4: NPTH, NPTH, F.Cu at (128.2, 110.7)
- added KiKit_MB_18_4: NPTH, NPTH, F.Cu at (81.5, 111.8)
- added KiKit_MB_18_5: NPTH, NPTH, F.Cu at (127.3, 110.7)
- added KiKit_MB_18_5: NPTH, NPTH, F.Cu at (80.7, 111.8)
- added KiKit_MB_18_6: NPTH, NPTH, F.Cu at (79.9, 111.8)
- added KiKit_MB_18_6: NPTH, NPTH, F.Cu at (126.5, 110.7)
- added KiKit_MB_18_7: NPTH, NPTH, F.Cu at (125.7, 110.7)
- added KiKit_MB_18_7: NPTH, NPTH, F.Cu at (79.0, 111.8)
- added KiKit_MB_19_1: NPTH, NPTH, F.Cu at (92.5, 99.5)
- added KiKit_MB_19_1: NPTH, NPTH, F.Cu at (139.1, 99.3)
- added KiKit_MB_19_2: NPTH, NPTH, F.Cu at (92.5, 98.7)
- added KiKit_MB_19_2: NPTH, NPTH, F.Cu at (139.1, 98.3)
- added KiKit_MB_19_3: NPTH, NPTH, F.Cu at (92.5, 97.9)
- added KiKit_MB_19_3: NPTH, NPTH, F.Cu at (139.1, 97.3)
- added KiKit_MB_19_4: NPTH, NPTH, F.Cu at (92.5, 97.1)
- added KiKit_MB_19_4: NPTH, NPTH, F.Cu at (139.1, 96.3)
- added KiKit_MB_19_5: NPTH, NPTH, F.Cu at (92.5, 96.3)
- added KiKit_MB_19_6: NPTH, NPTH, F.Cu at (92.5, 95.5)
- added KiKit_MB_1_1: NPTH, NPTH, F.Cu at (73.2, 74.3)
- added KiKit_MB_1_1: NPTH, NPTH, F.Cu at (119.8, 75.6)
- added KiKit_MB_1_2: NPTH, NPTH, F.Cu at (119.8, 74.6)
- added KiKit_MB_1_2: NPTH, NPTH, F.Cu at (73.2, 73.5)
- added KiKit_MB_1_3: NPTH, NPTH, F.Cu at (73.2, 72.7)
- added KiKit_MB_1_3: NPTH, NPTH, F.Cu at (119.8, 73.6)
- added KiKit_MB_1_4: NPTH, NPTH, F.Cu at (73.2, 71.9)
- added KiKit_MB_1_4: NPTH, NPTH, F.Cu at (119.8, 72.6)
- added KiKit_MB_1_5: NPTH, NPTH, F.Cu at (73.2, 71.1)
- added KiKit_MB_1_6: NPTH, NPTH, F.Cu at (73.2, 70.3)
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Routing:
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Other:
- board size 100.9 x 93.6 mm -> 101 x 93.6 mm
